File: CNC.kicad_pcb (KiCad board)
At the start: 2 copper layers, 100.3 x 90.2 mm, 40 parts, among them J1 Conn_01x02_Male, J2 Conn_01x01_Male, J3 SD-MODULE, J4 Micro_SD_Card, J5 UART0, J6 EXTRA1, U1 LM7805_TO220, U2 ESP32_DEVKITV1, U3 Z - TMC2209 BTT v1.2, U4 X - TMC2209 BTT v1.2, U5 A - TMC2209 BTT v1.2, U6 Y - TMC2209 BTT v1.2

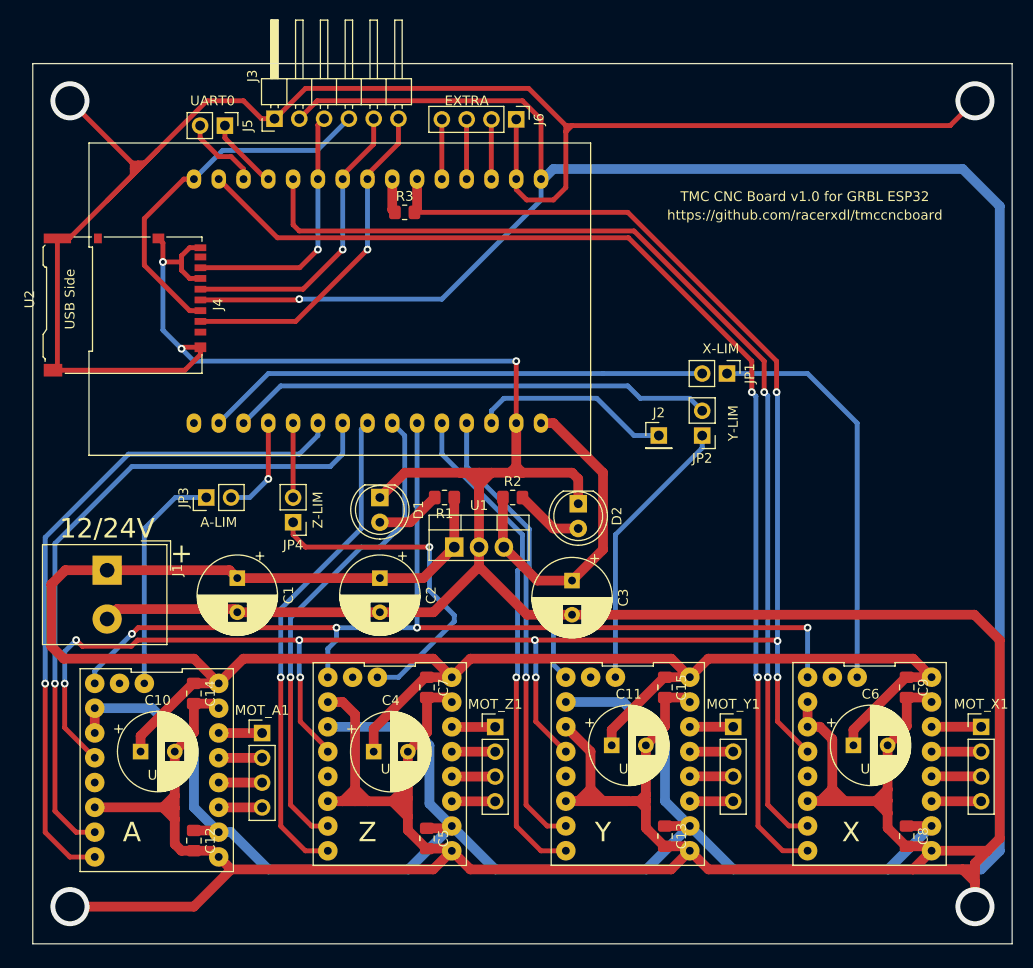
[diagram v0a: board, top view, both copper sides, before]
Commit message: Add preliminary gerber files
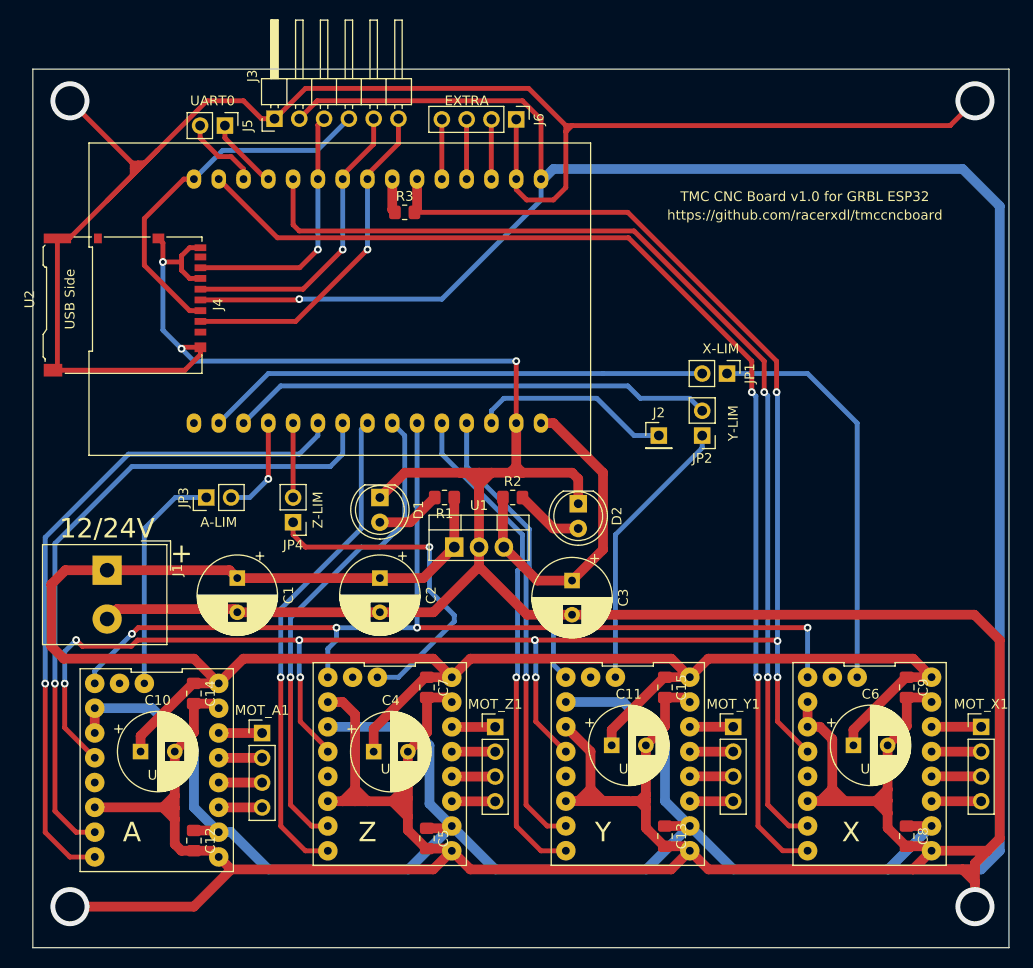
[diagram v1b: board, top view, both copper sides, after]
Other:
- board size 100.3 x 90.2 mm -> 100 x 90 mm
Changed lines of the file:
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@@
       (outputformat 1)
       (mirror false)
-      (drillshape 1)
+      (drillshape 0)
       (scaleselection 1)
-      (outputdirectory "")
+      (outputdirectory "Gerber/")
     )
   )
@@
     (fp_line (start -1 -0.625) (end 1 -0.625) (layer "F.Fab") (width 0.1))
     (fp_line (start -1 0.625) (end -1 -0.625) (layer "F.Fab") (width 0.1))
-    (pad "1" smd roundrect locked (at -1.0375 0 270) (size 1.175 1.45) (layers "F.Cu" "F.Paste" "F.Mask") (roundrect_rratio 0.212766)
+    (pad "1" smd roundrect locked (at -1.0375 0 270) (size 1.175 1.45) (layers "F.Cu" "F.Paste" "F.Mask") (roundrect_rratio 0.2127659574)
       (net 1 "+24V") (pintype "passive"))
-    (pad "2" smd roundrect locked (at 1.0375 0 270) (size 1.175 1.45) (layers "F.Cu" "F.Paste" "F.Mask") (roundrect_rratio 0.212766)
+    (pad "2" smd roundrect locked (at 1.0375 0 270) (size 1.175 1.45) (layers "F.Cu" "F.Paste" "F.Mask") (roundrect_rratio 0.2127659574)
       (net 2 "GND") (pintype "passive"))
     (model "${KICAD6_3DMODEL_DIR}/Capacitor_SMD.3dshapes/C_0805_2012Metric.wrl"
@@
     (fp_line (start -1 0.625) (end -1 -0.625) (layer "F.Fab") (width 0.1))
     (fp_line (start 1 -0.625) (end 1 0.625) (layer "F.Fab") (width 0.1))
-    (pad "1" smd roundrect locked (at -1 0) (size 1.2 1.4) (layers "F.Cu" "F.Paste" "F.Mask") (roundrect_rratio 0.208333)
+    (pad "1" smd roundrect locked (at -1 0) (size 1.2 1.4) (layers "F.Cu" "F.Paste" "F.Mask") (roundrect_rratio 0.2083333333)
       (net 31 "Net-(R3-Pad1)") (pintype "passive"))
-    (pad "2" smd roundrect locked (at 1 0) (size 1.2 1.4) (layers "F.Cu" "F.Paste" "F.Mask") (roundrect_rratio 0.208333)
+    (pad "2" smd roundrect locked (at 1 0) (size 1.2 1.4) (layers "F.Cu" "F.Paste" "F.Mask") (roundrect_rratio 0.2083333333)
       (net 32 "MOT_UART") (pintype "passive"))
     (model "${KICAD6_3DMODEL_DIR}/Resistor_SMD.3dshapes/R_0805_2012Metric.wrl"
@@
     (fp_line (start 1 0.625) (end -1 0.625) (layer "F.Fab") (width 0.1))
     (fp_line (start -1 0.625) (end -1 -0.625) (layer "F.Fab") (width 0.1))
-    (pad "1" smd roundrect locked (at -1.0375 0 270) (size 1.175 1.45) (layers "F.Cu" "F.Paste" "F.Mask") (roundrect_rratio 0.212766)
+    (pad "1" smd roundrect locked (at -1.0375 0 270) (size 1.175 1.45) (layers "F.Cu" "F.Paste" "F.Mask") (roundrect_rratio 0.2127659574)
       (net 4 "+3V3") (pintype "passive"))
-    (pad "2" smd roundrect locked (at 1.0375 0 270) (size 1.175 1.45) (layers "F.Cu" "F.Paste" "F.Mask") (roundrect_rratio 0.212766)
+    (pad "2" smd roundrect locked (at 1.0375 0 270) (size 1.175 1.45) (layers "F.Cu" "F.Paste" "F.Mask") (roundrect_rratio 0.2127659574)
       (net 2 "GND") (pintype "passive"))
     (model "${KICAD6_3DMODEL_DIR}/Capacitor_SMD.3dshapes/C_0805_2012Metric.wrl"
@@
     (fp_line (start 1 0.625) (end -1 0.625) (layer "F.Fab") (width 0.1))
     (fp_line (start -1 -0.625) (end 1 -0.625) (layer "F.Fab") (width 0.1))
-    (pad "1" smd roundrect locked (at -1.0375 0 270) (size 1.175 1.45) (layers "F.Cu" "F.Paste" "F.Mask") (roundrect_rratio 0.212766)
+    (pad "1" smd roundrect locked (at -1.0375 0 270) (size 1.175 1.45) (layers "F.Cu" "F.Paste" "F.Mask") (roundrect_rratio 0.2127659574)
       (net 4 "+3V3") (pintype "passive"))
-    (pad "2" smd roundrect locked (at 1.0375 0 270) (size 1.175 1.45) (layers "F.Cu" "F.Paste" "F.Mask") (roundrect_rratio 0.212766)
+    (pad "2" smd roundrect locked (at 1.0375 0 270) (size 1.175 1.45) (layers "F.Cu" "F.Paste" "F.Mask") (roundrect_rratio 0.2127659574)
       (net 2 "GND") (pintype "passive"))
     (model "${KICAD6_3DMODEL_DIR}/Capacitor_SMD.3dshapes/C_0805_2012Metric.wrl"
@@
     (fp_line (start -1 -0.625) (end 1 -0.625) (layer "F.Fab") (width 0.1))
     (fp_line (start -1 0.625) (end -1 -0.625) (layer "F.Fab") (width 0.1))
-    (pad "1" smd roundrect locked (at -1 0 180) (size 1.2 1.4) (layers "F.Cu" "F.Paste" "F.Mask") (roundrect_rratio 0.208333)
+    (pad "1" smd roundrect locked (at -1 0 180) (size 1.2 1.4) (layers "F.Cu" "F.Paste" "F.Mask") (roundrect_rratio 0.2083333333)
       (net 1 "+24V") (pintype "passive"))
-    (pad "2" smd roundrect locked (at 1 0 180) (size 1.2 1.4) (layers "F.Cu" "F.Paste" "F.Mask") (roundrect_rratio 0.208333)
+    (pad "2" smd roundrect locked (at 1 0 180) (size 1.2 1.4) (layers "F.Cu" "F.Paste" "F.Mask") (roundrect_rratio 0.2083333333)
       (net 5 "Net-(D1-Pad2)") (pintype "passive"))
     (model "${KICAD6_3DMODEL_DIR}/Resistor_SMD.3dshapes/R_0805_2012Metric.wrl"
@@
     (fp_line (start 1 0.625) (end -1 0.625) (layer "F.Fab") (width 0.1))
     (fp_line (start -1 0.625) (end -1 -0.625) (layer "F.Fab") (width 0.1))
-    (pad "1" smd roundrect locked (at -1.0375 0 270) (size 1.175 1.45) (layers "F.Cu" "F.Paste" "F.Mask") (roundrect_rratio 0.212766)
+    (pad "1" smd roundrect locked (at -1.0375 0 270) (size 1.175 1.45) (layers "F.Cu" "F.Paste" "F.Mask") (roundrect_rratio 0.2127659574)
       (net 1 "+24V") (pintype "passive"))
-    (pad "2" smd roundrect locked (at 1.0375 0 270) (size 1.175 1.45) (layers "F.Cu" "F.Paste" "F.Mask") (roundrect_rratio 0.212766)
+    (pad "2" smd roundrect locked (at 1.0375 0 270) (size 1.175 1.45) (layers "F.Cu" "F.Paste" "F.Mask") (roundrect_rratio 0.2127659574)
       (net 2 "GND") (pintype "passive"))
     (model "${KICAD6_3DMODEL_DIR}/Capacitor_SMD.3dshapes/C_0805_2012Metric.wrl"
@@
     (fp_line (start -1 -0.625) (end 1 -0.625) (layer "F.Fab") (width 0.1))
     (fp_line (start 1 0.625) (end -1 0.625) (layer "F.Fab") (width 0.1))
-    (pad "1" smd roundrect locked (at -1.0375 0 270) (size 1.175 1.45) (layers "F.Cu" "F.Paste" "F.Mask") (roundrect_rratio 0.212766)
+    (pad "1" smd roundrect locked (at -1.0375 0 270) (size 1.175 1.45) (layers "F.Cu" "F.Paste" "F.Mask") (roundrect_rratio 0.2127659574)
       (net 4 "+3V3") (pintype "passive"))
-    (pad "2" smd roundrect locked (at 1.0375 0 270) (size 1.175 1.45) (layers "F.Cu" "F.Paste" "F.Mask") (roundrect_rratio 0.212766)
+    (pad "2" smd roundrect locked (at 1.0375 0 270) (size 1.175 1.45) (layers "F.Cu" "F.Paste" "F.Mask") (roundrect_rratio 0.2127659574)
       (net 2 "GND") (pintype "passive"))
     (model "${KICAD6_3DMODEL_DIR}/Capacitor_SMD.3dshapes/C_0805_2012Metric.wrl"
@@
     (fp_line (start 1 -0.625) (end 1 0.625) (layer "F.Fab") (width 0.1))
     (fp_line (start 1 0.625) (end -1 0.625) (layer "F.Fab") (width 0.1))
-    (pad "1" smd roundrect locked (at -1.0375 0 270) (size 1.175 1.45) (layers "F.Cu" "F.Paste" "F.Mask") (roundrect_rratio 0.212766)
+    (pad "1" smd roundrect locked (at -1.0375 0 270) (size 1.175 1.45) (layers "F.Cu" "F.Paste" "F.Mask") (roundrect_rratio 0.2127659574)
       (net 1 "+24V") (pintype "passive"))
-    (pad "2" smd roundrect locked (at 1.0375 0 270) (size 1.175 1.45) (layers "F.Cu" "F.Paste" "F.Mask") (roundrect_rratio 0.212766)
+    (pad "2" smd roundrect locked (at 1.0375 0 270) (size 1.175 1.45) (layers "F.Cu" "F.Paste" "F.Mask") (roundrect_rratio 0.2127659574)
       (net 2 "GND") (pintype "passive"))
     (model "${KICAD6_3DMODEL_DIR}/Capacitor_SMD.3dshapes/C_0805_2012Metric.wrl"
@@
     (fp_line (start -1 -0.625) (end 1 -0.625) (layer "F.Fab") (width 0.1))
     (fp_line (start 1 0.625) (end -1 0.625) (layer "F.Fab") (width 0.1))
-    (pad "1" smd roundrect locked (at -1 0) (size 1.2 1.4) (layers "F.Cu" "F.Paste" "F.Mask") (roundrect_rratio 0.208333)
+    (pad "1" smd roundrect locked (at -1 0) (size 1.2 1.4) (layers "F.Cu" "F.Paste" "F.Mask") (roundrect_rratio 0.2083333333)
       (net 3 "+5V") (pintype "passive"))
-    (pad "2" smd roundrect locked (at 1 0) (size 1.2 1.4) (layers "F.Cu" "F.Paste" "F.Mask") (roundrect_rratio 0.208333)
+    (pad "2" smd roundrect locked (at 1 0) (size 1.2 1.4) (layers "F.Cu" "F.Paste" "F.Mask") (roundrect_rratio 0.2083333333)
       (net 6 "Net-(D2-Pad2)") (pintype "passive"))
     (model "${KICAD6_3DMODEL_DIR}/Resistor_SMD.3dshapes/R_0805_2012Metric.wrl"
@@
     (fp_line (start 1 -0.625) (end 1 0.625) (layer "F.Fab") (width 0.1))
     (fp_line (start 1 0.625) (end -1 0.625) (layer "F.Fab") (width 0.1))
-    (pad "1" smd roundrect locked (at -1.0375 0 270) (size 1.175 1.45) (layers "F.Cu" "F.Paste" "F.Mask") (roundrect_rratio 0.212766)
+    (pad "1" smd roundrect locked (at -1.0375 0 270) (size 1.175 1.45) (layers "F.Cu" "F.Paste" "F.Mask") (roundrect_rratio 0.2127659574)
       (net 1 "+24V") (pintype "passive"))
-    (pad "2" smd roundrect locked (at 1.0375 0 270) (size 1.175 1.45) (layers "F.Cu" "F.Paste" "F.Mask") (roundrect_rratio 0.212766)
+    (pad "2" smd roundrect locked (at 1.0375 0 270) (size 1.175 1.45) (layers "F.Cu" "F.Paste" "F.Mask") (roundrect_rratio 0.2127659574)
       (net 2 "GND") (pintype "passive"))
     (model "${KICAD6_3DMODEL_DIR}/Capacitor_SMD.3dshapes/C_0805_2012Metric.wrl"
@@
     (fp_line (start 1 0.625) (end -1 0.625) (layer "F.Fab") (width 0.1))
     (fp_line (start -1 -0.625) (end 1 -0.625) (layer "F.Fab") (width 0.1))
-    (pad "1" smd roundrect locked (at -1.0375 0 270) (size 1.175 1.45) (layers "F.Cu" "F.Paste" "F.Mask") (roundrect_rratio 0.212766)
+    (pad "1" smd roundrect locked (at -1.0375 0 270) (size 1.175 1.45) (layers "F.Cu" "F.Paste" "F.Mask") (roundrect_rratio 0.2127659574)
       (net 4 "+3V3") (pintype "passive"))
-    (pad "2" smd roundrect locked (at 1.0375 0 270) (size 1.175 1.45) (layers "F.Cu" "F.Paste" "F.Mask") (roundrect_rratio 0.212766)
+    (pad "2" smd roundrect locked (at 1.0375 0 270) (size 1.175 1.45) (layers "F.Cu" "F.Paste" "F.Mask") (roundrect_rratio 0.2127659574)
       (net 2 "GND") (pintype "passive"))
     (model "${KICAD6_3DMODEL_DIR}/Capacitor_SMD.3dshapes/C_0805_2012Metric.wrl"
@@
     )
   )
-  (gr_rect (start 98.99548 54.432865) (end 199.32548 144.602865) (layer "Edge.Cuts") (width 0.1) (fill none))
+  (gr_rect (start 99 55) (end 199 145) (layer "Edge.Cuts") (width 0.1) (fill none))
   (gr_text "Y" (at 157.41548 133.172865) (layer "F.SilkS")
     (effects (font (size 2 2) (thickness 0.15)))
